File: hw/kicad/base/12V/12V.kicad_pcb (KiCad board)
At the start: 2 copper layers, 50 x 50 mm, 29 parts, among them J1 USB_B_Micro, J2 TOP, J3 XT60PW-M, J4 BUTTOM, U1 LM1117MP-3.3, U2 LM2596S-5, U3 CP2102N-Axx-xQFN28

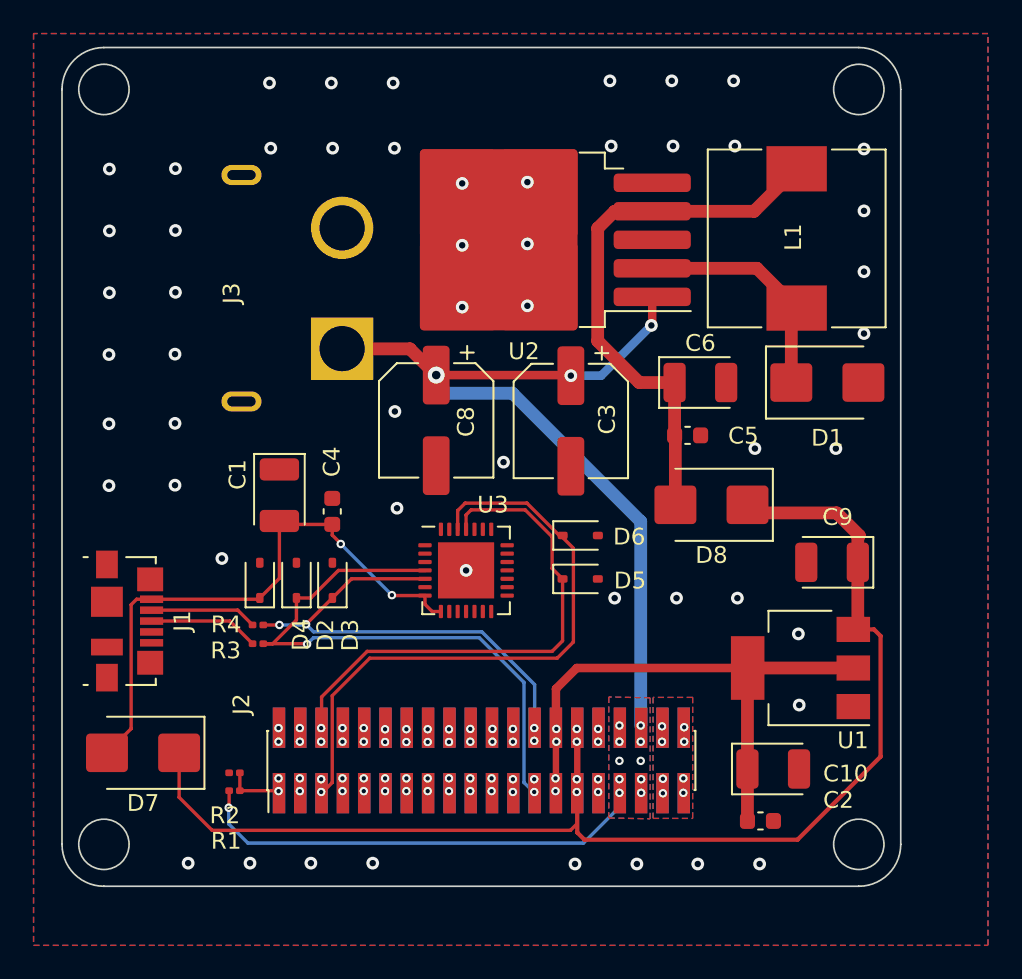
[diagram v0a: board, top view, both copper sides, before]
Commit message: 修改尺寸至45x45
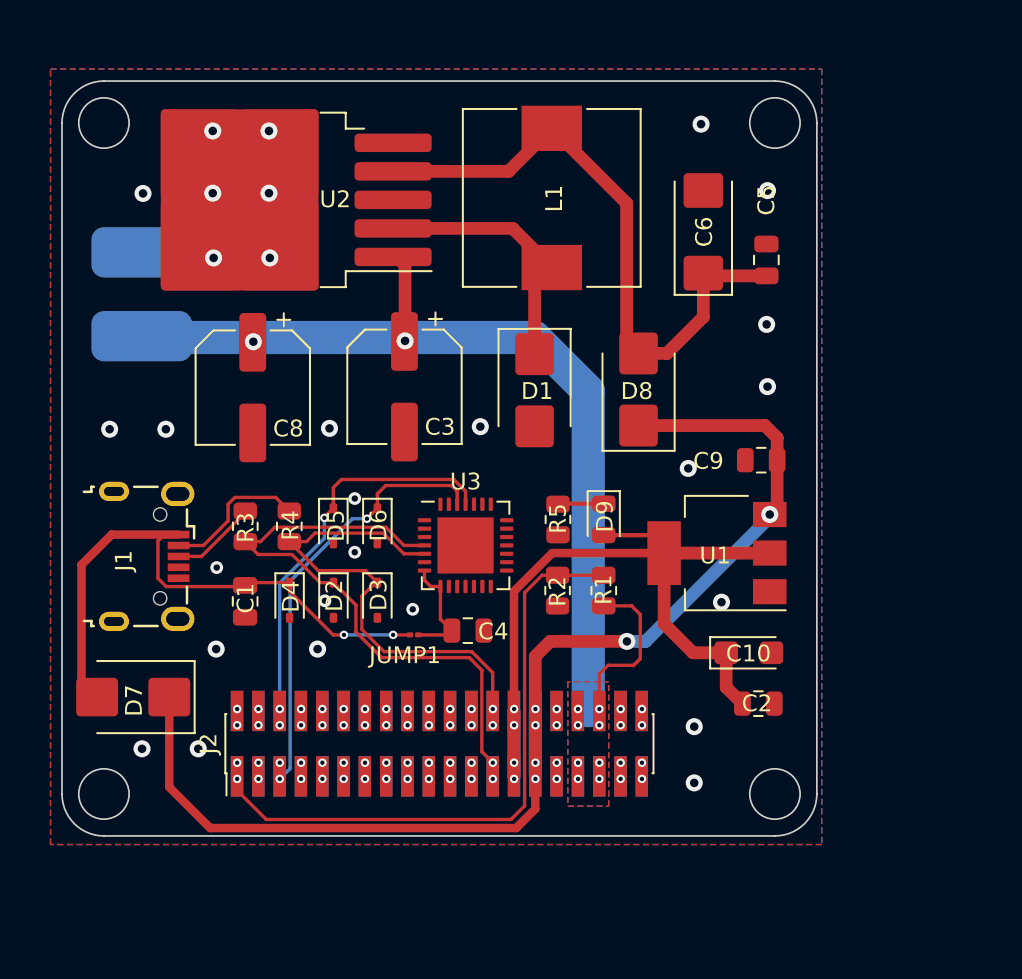
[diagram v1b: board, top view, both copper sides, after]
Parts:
- added D9: LED, LED_SMD:LED_0805_2012Metric, F.Cu at (83.0, 58.8)
- added JUMP1: 0, Resistor_SMD:R_01005_0402Metric, F.Cu at (71.7, 65.7)
- added R5: 10k, Resistor_SMD:R_0805_2012Metric, F.Cu at (80.3, 58.9)
- C1: footprint Capacitor_Tantalum_SMD:CP_EIA-3528-21_Kemet-B -> Capacitor_SMD:C_0805_2012Metric
- C10: value 10uF -> 47uF; footprint Capacitor_Tantalum_SMD:CP_EIA-3528-21_Kemet-B -> Capacitor_Tantalum_SMD:CP_EIA-3216-12_Kemet-S
- C2, C4, C5: footprint Capacitor_SMD:C_0603_1608Metric -> Capacitor_SMD:C_0805_2012Metric
- C6: footprint Capacitor_Tantalum_SMD:CP_EIA-3528-21_Kemet-B -> Capacitor_Tantalum_SMD:CP_EIA-6032-28_Kemet-C
- C9: value 10uF -> 0.1uF; footprint Capacitor_Tantalum_SMD:CP_EIA-3528-21_Kemet-B -> Capacitor_SMD:C_0805_2012Metric
- J1: footprint Connector_USB:USB_Micro-B_Molex_47346-0001 -> Connector_USB:USB_Micro-B_Wuerth_629105150521
- J3: value XT60PW-M -> XT30PW-M; footprint XT:XT60-PW-M -> XT:XT30-PAD
- R1, R2, R3, R4: footprint Resistor_SMD:R_0201_0603Metric -> Resistor_SMD:R_0805_2012Metric
- moved R1 25.0 mm to (83.0, 63.1), turned to 90 degrees
- moved R2 22.1 mm to (80.3, 63.1), turned to -90 degrees
- moved D1 17.5 mm to (78.9, 51.1), turned to -90 degrees
- moved U2 15.6 mm to (62.8, 39.8)
- moved D5 15.1 mm to (66.9, 59.2), turned to -90 degrees
- moved L1 14.8 mm to (79.9, 39.7)
- moved D6 12.1 mm to (69.5, 59.2), turned to -90 degrees
- moved J3 11.9 mm to (49.6, 45.4)
- moved C5 11.5 mm to (92.7, 43.4), turned to 90 degrees
- moved C8 11.1 mm to (62.1, 51.0)
- moved C4 10.8 mm to (74.9, 65.5), turned to 180 degrees
- moved C3 10.1 mm to (71.1, 50.9)
- moved C6 8.99 mm to (89.0, 41.7), turned to 90 degrees
- moved U1 8.47 mm to (89.8, 60.9)
- moved D8 8.13 mm to (85.1, 51.1), turned to 90 degrees
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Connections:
- C4 pad 2: VBUS -> Net-(U3-VBUS)
- J3 pad 1: +BATT -> GND
- J3 pad 2: GND -> +BATT
- U3 pad 7: VBUS -> Net-(U3-VBUS)
- U3 pad 8: VBUS -> Net-(U3-VBUS)
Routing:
- net /ADC_1: track 3.38 -> 36.9 mm
- net +BATT: track 78.4 -> 62.1 mm, vias 14 -> 10
- net +3.3V: track 33.5 -> 46.7 mm
- net /UART1_RX: track 36.7 -> 25.8 mm, vias 2 -> 3
- net Net-(D1-K): track 14.2 -> 21.5 mm
- net /UART1_TX: track 30.8 -> 23.8 mm, vias 2 -> 3
- net Net-(U3-VBUS): track 0.00 -> 6.70 mm
- net +5V: track 77.8 -> 72.6 mm, vias 4 -> 6
- net Net-(D8-A): track 33.0 -> 37.3 mm
- net Net-(D9-K): track 0.00 -> 2.74 mm
- net Net-(J1-D-): track 6.39 -> 8.70 mm
- net Net-(J1-D+): track 6.58 -> 5.15 mm
- net /USB-: track 28.5 -> 29.4 mm, vias 4 -> 2
- net /USB+: track 35.9 -> 36.3 mm, vias 3 -> 2
- net GND: vias 66 -> 40
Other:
- board size 50 x 50 mm -> 45 x 45 mm
